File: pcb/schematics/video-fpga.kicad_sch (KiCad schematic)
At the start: 42 parts, among them U4 LCMXO2-7000HC-4TG144C, X1 ASV-xxxMHz

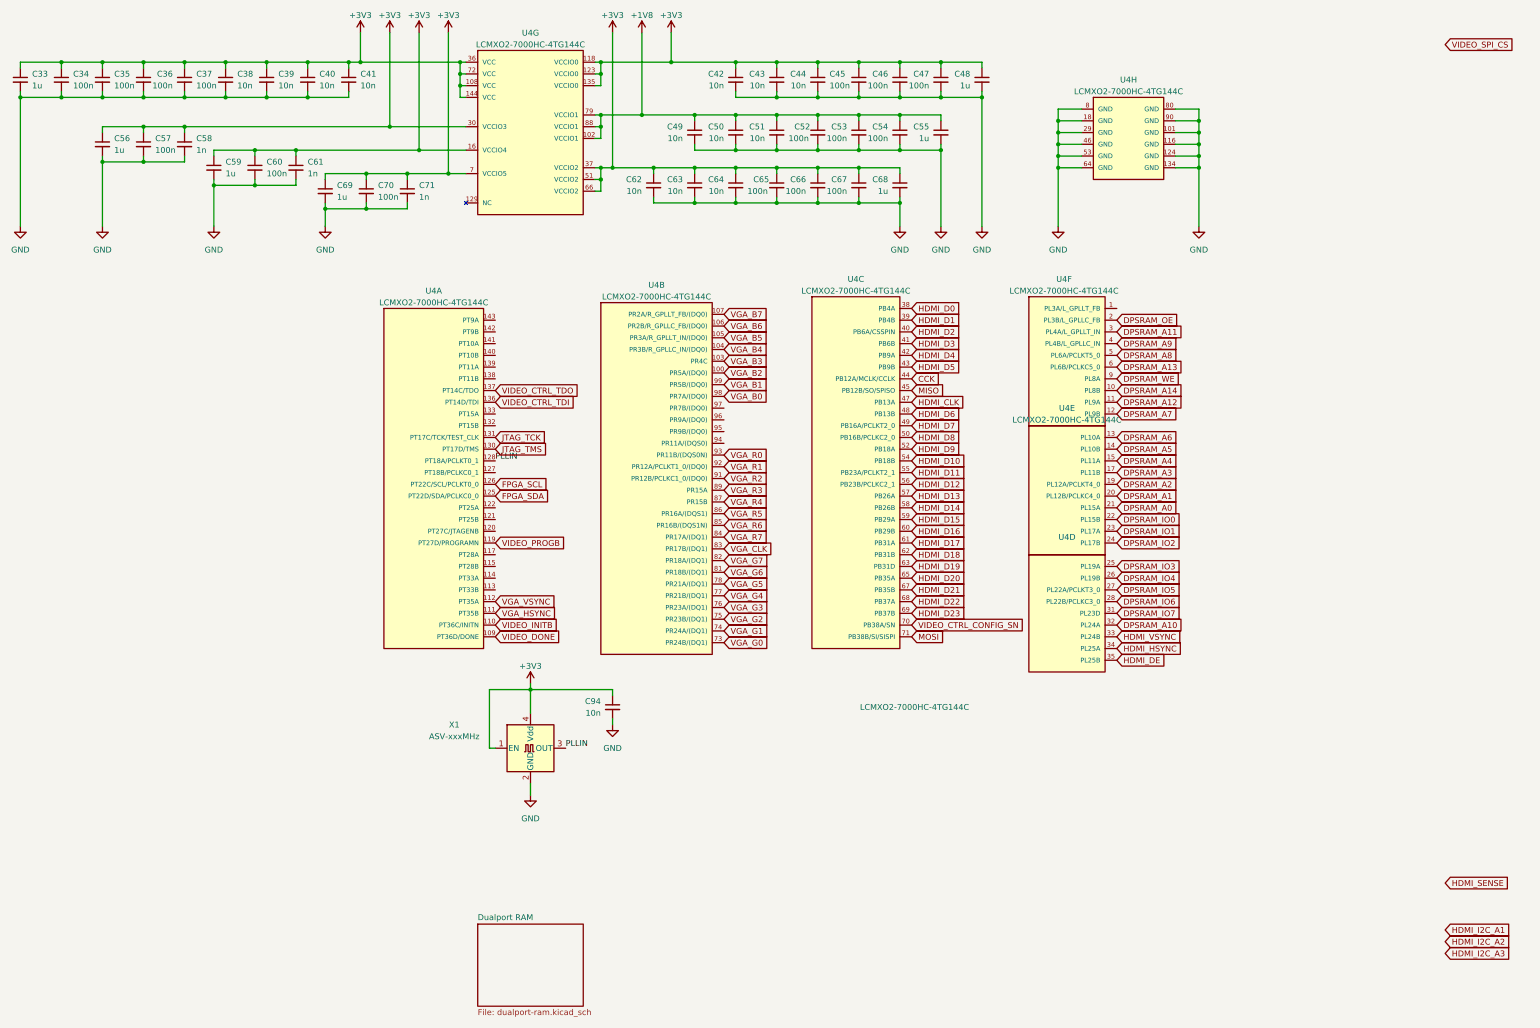
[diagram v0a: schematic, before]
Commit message: add shield
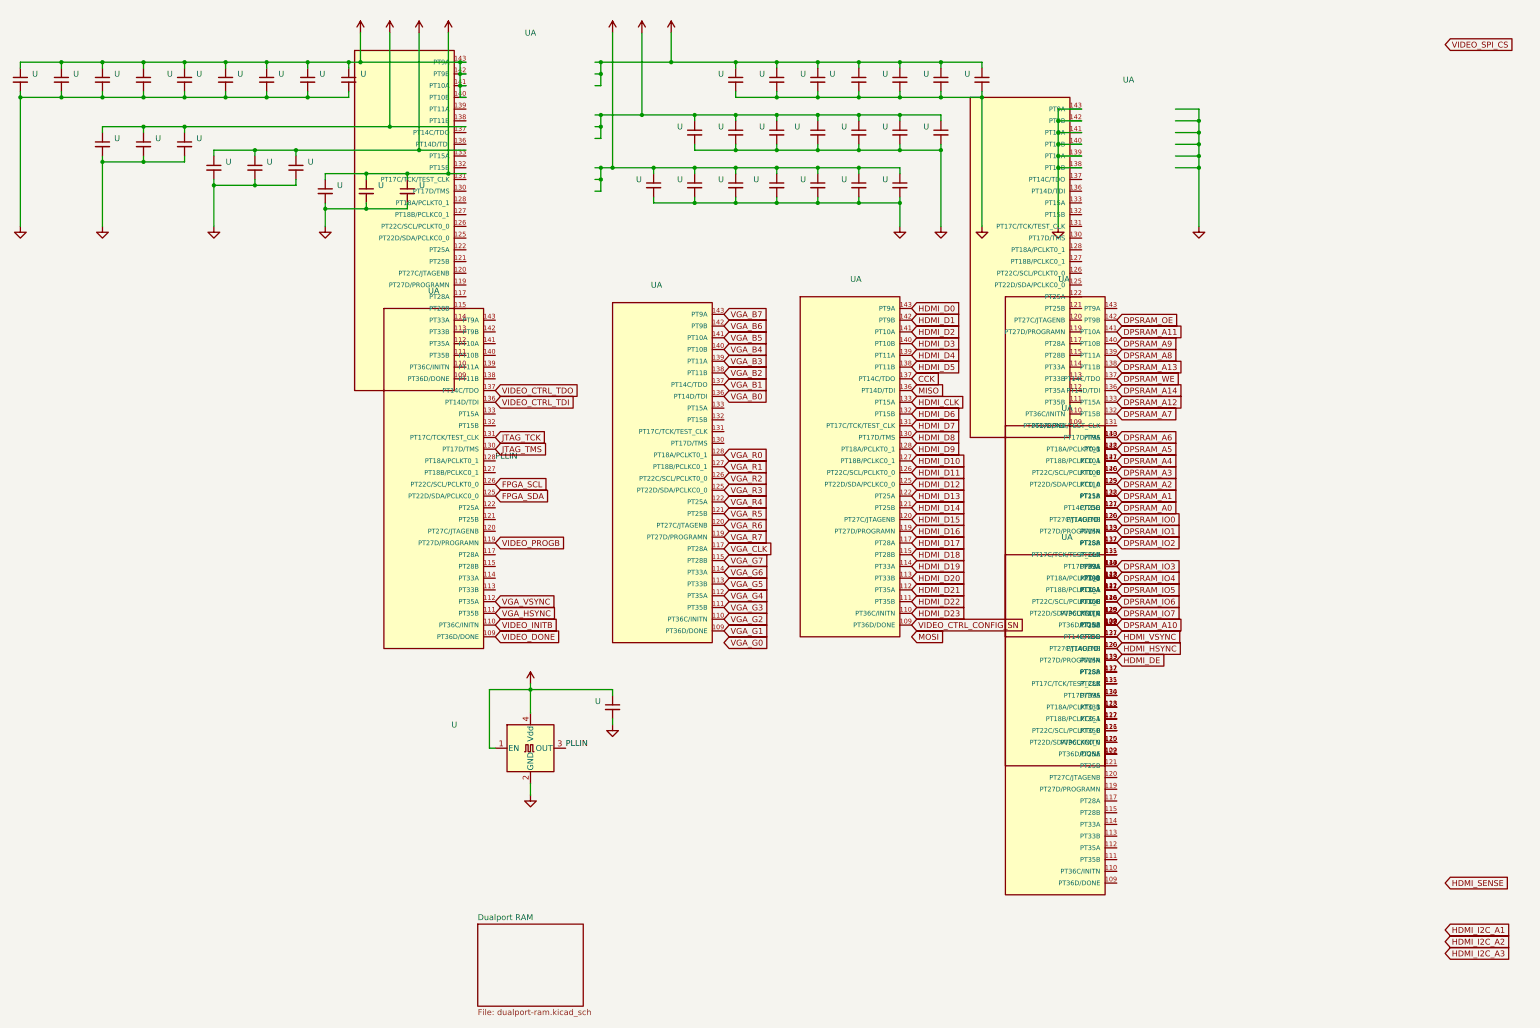
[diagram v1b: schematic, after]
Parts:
- U: renamed from C67; value 100n -> (none); footprint Capacitor_SMD:C_0603_1608Metric -> (none)
- U: renamed from U4; value LCMXO2-7000HC-4TG144C -> (none); footprint LCMXO2-7000HC-4TG144C:Lattice_Semiconductor-LCMXO2-7000HC-4TG144C-Level_C -> (none)
- U: renamed from C64; value 10n -> (none); footprint Capacitor_SMD:C_0402_1005Metric -> (none)
- U: renamed from C52; value 100n -> (none); footprint Capacitor_SMD:C_0603_1608Metric -> (none)
- U: renamed from C57; value 100n -> (none); footprint Capacitor_SMD:C_0603_1608Metric -> (none)
- U: renamed from C66; value 100n -> (none); footprint Capacitor_SMD:C_0603_1608Metric -> (none)
- U: renamed from C63; value 10n -> (none); footprint Capacitor_SMD:C_0402_1005Metric -> (none)
- U: renamed from C33; value 1u -> (none); footprint Capacitor_SMD:C_0805_2012Metric -> (none)
- U: renamed from C42; value 10n -> (none); footprint Capacitor_SMD:C_0402_1005Metric -> (none)
- U: renamed from C43; value 10n -> (none); footprint Capacitor_SMD:C_0402_1005Metric -> (none)
- U: renamed from C37; value 100n -> (none); footprint Capacitor_SMD:C_0603_1608Metric -> (none)
- U: renamed from C55; value 1u -> (none); footprint Capacitor_SMD:C_0805_2012Metric -> (none)
- U: renamed from C71; value 1n -> (none); footprint Capacitor_SMD:C_0402_1005Metric -> (none)
- U: renamed from C41; value 10n -> (none); footprint Capacitor_SMD:C_0402_1005Metric -> (none)
- U: renamed from C48; value 1u -> (none); footprint Capacitor_SMD:C_0805_2012Metric -> (none)
- U: renamed from C61; value 1n -> (none); footprint Capacitor_SMD:C_0402_1005Metric -> (none)
- U: renamed from C35; value 100n -> (none); footprint Capacitor_SMD:C_0603_1608Metric -> (none)
- U: renamed from C56; value 1u -> (none); footprint Capacitor_SMD:C_0805_2012Metric -> (none)
- U: renamed from C34; value 100n -> (none); footprint Capacitor_SMD:C_0603_1608Metric -> (none)
- U: renamed from C53; value 100n -> (none); footprint Capacitor_SMD:C_0603_1608Metric -> (none)
- U: renamed from C51; value 10n -> (none); footprint Capacitor_SMD:C_0402_1005Metric -> (none)
- U: renamed from C58; value 1n -> (none); footprint Capacitor_SMD:C_0402_1005Metric -> (none)
- U: renamed from C44; value 10n -> (none); footprint Capacitor_SMD:C_0402_1005Metric -> (none)
- U: renamed from C49; value 10n -> (none); footprint Capacitor_SMD:C_0402_1005Metric -> (none)
- U: renamed from C60; value 100n -> (none); footprint Capacitor_SMD:C_0603_1608Metric -> (none)
- U: renamed from C39; value 10n -> (none); footprint Capacitor_SMD:C_0402_1005Metric -> (none)
- U: renamed from C36; value 100n -> (none); footprint Capacitor_SMD:C_0603_1608Metric -> (none)
- U: renamed from C50; value 10n -> (none); footprint Capacitor_SMD:C_0402_1005Metric -> (none)
- U: renamed from C69; value 1u -> (none); footprint Capacitor_SMD:C_0805_2012Metric -> (none)
- U: renamed from C54; value 100n -> (none); footprint Capacitor_SMD:C_0603_1608Metric -> (none)
- U: renamed from C59; value 1u -> (none); footprint Capacitor_SMD:C_0805_2012Metric -> (none)
- U: renamed from C45; value 100n -> (none); footprint Capacitor_SMD:C_0603_1608Metric -> (none)
- U: renamed from C70; value 100n -> (none); footprint Capacitor_SMD:C_0603_1608Metric -> (none)
- U: renamed from C38; value 10n -> (none); footprint Capacitor_SMD:C_0402_1005Metric -> (none)
- U: renamed from C94; value 10n -> (none); footprint Capacitor_SMD:C_0402_1005Metric -> (none)
- U: renamed from X1; value ASV-xxxMHz -> (none); footprint Oscillator:Oscillator_SMD_Abracon_ASV-4Pin_7.0x5.1mm -> (none)
- U: renamed from C40; value 10n -> (none); footprint Capacitor_SMD:C_0402_1005Metric -> (none)
- U: renamed from C65; value 100n -> (none); footprint Capacitor_SMD:C_0603_1608Metric -> (none)
- U: renamed from C68; value 1u -> (none); footprint Capacitor_SMD:C_0805_2012Metric -> (none)
- U: renamed from C46; value 100n -> (none); footprint Capacitor_SMD:C_0603_1608Metric -> (none)
- U: renamed from C62; value 10n -> (none); footprint Capacitor_SMD:C_0402_1005Metric -> (none)
- U: renamed from C47; value 100n -> (none); footprint Capacitor_SMD:C_0603_1608Metric -> (none)
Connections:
- net +1V8: no longer U.102 (VCCIO1), U.79 (VCCIO1), U.88 (VCCIO1)
- net +3V3: now also U.140 (PT10B), U.141 (PT10A), U.142 (PT9B), U.143 (PT9A); no longer U.108 (VCC), U.118 (VCCIO0), U.123 (VCCIO0), U.135 (VCCIO0), U.144 (VCC), U.16 (VCCIO4), U.30 (VCCIO3), U.36 (VCC), U.37 (VCCIO2), U.51 (VCCIO2), U.66 (VCCIO2), U.7 (VCCIO5), U.72 (VCC)
- net CCK: now also U.137 (PT14C/TDO); no longer U.44 (PB12A/MCLK/CCLK)
- net DPSRAM_A0: now also U.121 (PT25B), U.137 (PT14C/TDO); no longer U.21 (PL15A)
- net DPSRAM_A1: now also U.122 (PT25A), U.138 (PT11B); no longer U.20 (PL12B/PCLKC4_0)
- net DPSRAM_A10: now also U.109 (PT36D/DONE), U.122 (PT25A), U.138 (PT11B); no longer U.32 (PL24A)
- net DPSRAM_A11: now also U.141 (PT10A); no longer U.3 (PL4A/L_GPLLT_IN)
- net DPSRAM_A12: now also U.133 (PT15A); no longer U.11 (PL9A)
- net DPSRAM_A13: now also U.138 (PT11B); no longer U.6 (PL6B/PCLKC5_0)
- net DPSRAM_A14: now also U.136 (PT14D/TDI); no longer U.10 (PL8B)
- net DPSRAM_A2: now also U.125 (PT22D/SDA/PCLKC0_0), U.139 (PT11A); no longer U.19 (PL12A/PCLKT4_0)
- net DPSRAM_A3: now also U.126 (PT22C/SCL/PCLKT0_0), U.140 (PT10B); no longer U.17 (PL11B)
- net DPSRAM_A4: now also U.127 (PT18B/PCLKC0_1), U.141 (PT10A); no longer U.15 (PL11A)
- net DPSRAM_A5: now also U.128 (PT18A/PCLKT0_1), U.142 (PT9B); no longer U.14 (PL10B)
- net DPSRAM_A6: now also U.130 (PT17D/TMS), U.143 (PT9A); no longer U.13 (PL10A)
- net DPSRAM_A7: now also U.132 (PT15B); no longer U.12 (PL9B)
- net DPSRAM_A8: now also U.139 (PT11A); no longer U.5 (PL6A/PCLKT5_0)
- net DPSRAM_A9: now also U.140 (PT10B); no longer U.4 (PL4B/L_GPLLC_IN)
- net DPSRAM_IO0: now also U.120 (PT27C/JTAGENB), U.136 (PT14D/TDI); no longer U.22 (PL15B)
- net DPSRAM_IO1: now also U.119 (PT27D/PROGRAMN), U.133 (PT15A); no longer U.23 (PL17A)
- net DPSRAM_IO2: now also U.117 (PT28A), U.132 (PT15B); no longer U.24 (PL17B)
- net DPSRAM_IO3: now also U.114 (PT33A), U.130 (PT17D/TMS), U.143 (PT9A); no longer U.25 (PL19A)
- net DPSRAM_IO4: now also U.113 (PT33B), U.128 (PT18A/PCLKT0_1), U.142 (PT9B); no longer U.26 (PL19B)
- net DPSRAM_IO5: now also U.112 (PT35A), U.127 (PT18B/PCLKC0_1), U.141 (PT10A); no longer U.27 (PL22A/PCLKT3_0)
- net DPSRAM_IO6: now also U.111 (PT35B), U.126 (PT22C/SCL/PCLKT0_0), U.140 (PT10B); no longer U.28 (PL22B/PCLKC3_0)
- net DPSRAM_IO7: now also U.110 (PT36C/INITN), U.125 (PT22D/SDA/PCLKC0_0), U.139 (PT11A); no longer U.31 (PL23D)
- net DPSRAM_OE: now also U.142 (PT9B); no longer U.2 (PL3B/L_GPLLC_FB)
- net DPSRAM_WE: now also U.137 (PT14C/TDO); no longer U.9 (PL8A)
- net GND: now also U.138 (PT11B), U.139 (PT11A), U.140 (PT10B), U.141 (PT10A), U.142 (PT9B), U.143 (PT9A); no longer U.101 (GND), U.116 (GND), U.124 (GND), U.134 (GND), U.18 (GND), U.29 (GND), U.46 (GND), U.53 (GND), U.64 (GND), U.8 (GND), U.80 (GND), U.90 (GND)
- net HDMI_CLK: now also U.133 (PT15A); no longer U.47 (PB13A)
- net HDMI_D0: now also U.143 (PT9A); no longer U.38 (PB4A)
- net HDMI_D1: now also U.142 (PT9B); no longer U.39 (PB4B)
- net HDMI_D10: now also U.127 (PT18B/PCLKC0_1); no longer U.54 (PB18B)
- net HDMI_D11: now also U.126 (PT22C/SCL/PCLKT0_0); no longer U.55 (PB23A/PCLKT2_1)
- net HDMI_D12: now also U.125 (PT22D/SDA/PCLKC0_0); no longer U.56 (PB23B/PCLKC2_1)
- net HDMI_D13: now also U.122 (PT25A); no longer U.57 (PB26A)
- net HDMI_D14: now also U.121 (PT25B); no longer U.58 (PB26B)
- net HDMI_D15: now also U.120 (PT27C/JTAGENB); no longer U.59 (PB29A)
- net HDMI_D16: now also U.119 (PT27D/PROGRAMN); no longer U.60 (PB29B)
- net HDMI_D17: now also U.117 (PT28A); no longer U.61 (PB31A)
- net HDMI_D18: now also U.115 (PT28B); no longer U.62 (PB31B)
- net HDMI_D19: now also U.114 (PT33A); no longer U.63 (PB31D)
- net HDMI_D2: now also U.141 (PT10A); no longer U.40 (PB6A/CSSPIN)
- net HDMI_D20: now also U.113 (PT33B); no longer U.65 (PB35A)
- net HDMI_D21: now also U.112 (PT35A); no longer U.67 (PB35B)
- net HDMI_D22: now also U.111 (PT35B); no longer U.68 (PB37A)
- net HDMI_D23: now also U.110 (PT36C/INITN); no longer U.69 (PB37B)
- net HDMI_D3: now also U.140 (PT10B); no longer U.41 (PB6B)
- net HDMI_D4: now also U.139 (PT11A); no longer U.42 (PB9A)
- net HDMI_D5: now also U.138 (PT11B); no longer U.43 (PB9B)
- net HDMI_D6: now also U.132 (PT15B); no longer U.48 (PB13B)
- net HDMI_D7: now also U.131 (PT17C/TCK/TEST_CLK); no longer U.49 (PB16A/PCLKT2_0)
- net HDMI_D8: now also U.130 (PT17D/TMS); no longer U.50 (PB16B/PCLKC2_0)
- net HDMI_D9: now also U.128 (PT18A/PCLKT0_1); no longer U.52 (PB18A)
- net HDMI_DE: now also U.119 (PT27D/PROGRAMN), U.133 (PT15A); no longer U.35 (PL25B)
- net HDMI_HSYNC: now also U.120 (PT27C/JTAGENB), U.136 (PT14D/TDI); no longer U.34 (PL25A)
- net HDMI_VSYNC: now also U.121 (PT25B), U.137 (PT14C/TDO); no longer U.33 (PL24B)
- net MISO: now also U.136 (PT14D/TDI); no longer U.45 (PB12B/SO/SPISO)
- net MOSI: no longer U.71 (PB38B/SI/SISPI)
- net VGA_B0: now also U.136 (PT14D/TDI); no longer U.98 (PR7A/(DQ0))
- net VGA_B1: now also U.137 (PT14C/TDO); no longer U.99 (PR5B/(DQ0))
- net VGA_B2: now also U.138 (PT11B); no longer U.100 (PR5A/(DQ0))
- net VGA_B3: now also U.139 (PT11A); no longer U.103 (PR4C)
- net VGA_B4: now also U.140 (PT10B); no longer U.104 (PR3B/R_GPLLC_IN/(DQ0))
- net VGA_B5: now also U.141 (PT10A); no longer U.105 (PR3A/R_GPLLT_IN/(DQ0))
- net VGA_B6: now also U.142 (PT9B); no longer U.106 (PR2B/R_GPLLC_FB/(DQ0))
- net VGA_B7: now also U.143 (PT9A); no longer U.107 (PR2A/R_GPLLT_FB/(DQ0))
- net VGA_CLK: now also U.117 (PT28A); no longer U.83 (PR17B/(DQ1))
- net VGA_G0: no longer U.73 (PR24B/(DQ1))
- net VGA_G1: now also U.109 (PT36D/DONE); no longer U.74 (PR24A/(DQ1))
- net VGA_G2: now also U.110 (PT36C/INITN); no longer U.75 (PR23B/(DQ1))
- net VGA_G3: now also U.111 (PT35B); no longer U.76 (PR23A/(DQ1))
- net VGA_G4: now also U.112 (PT35A); no longer U.77 (PR21B/(DQ1))
- net VGA_G5: now also U.113 (PT33B); no longer U.78 (PR21A/(DQ1))
- net VGA_G6: now also U.114 (PT33A); no longer U.81 (PR18B/(DQ1))
- net VGA_G7: now also U.115 (PT28B); no longer U.82 (PR18A/(DQ1))
- net VGA_R0: now also U.128 (PT18A/PCLKT0_1); no longer U.93 (PR11B/(DQS0N))
- net VGA_R1: now also U.127 (PT18B/PCLKC0_1); no longer U.92 (PR12A/PCLKT1_0/(DQ0))
- net VGA_R2: now also U.126 (PT22C/SCL/PCLKT0_0); no longer U.91 (PR12B/PCLKC1_0/(DQ0))
- net VGA_R3: now also U.125 (PT22D/SDA/PCLKC0_0); no longer U.89 (PR15A)
- net VGA_R4: now also U.122 (PT25A); no longer U.87 (PR15B)
- net VGA_R5: now also U.121 (PT25B); no longer U.86 (PR16A/(DQS1))
- net VGA_R6: now also U.120 (PT27C/JTAGENB); no longer U.85 (PR16B/(DQS1N))
- net VGA_R7: now also U.119 (PT27D/PROGRAMN); no longer U.84 (PR17A/(DQ1))
- net VIDEO_CTRL_CONFIG_SN: now also U.109 (PT36D/DONE); no longer U.70 (PB38A/SN)
- new net: U.109 (PT36D/DONE), U.122 (PT25A)
- new net: U.110 (PT36C/INITN), U.125 (PT22D/SDA/PCLKC0_0)
- new net: U.111 (PT35B), U.126 (PT22C/SCL/PCLKT0_0)
- new net: U.112 (PT35A), U.127 (PT18B/PCLKC0_1)
- new net: U.113 (PT33B), U.128 (PT18A/PCLKT0_1)
- new net: U.114 (PT33A), U.130 (PT17D/TMS)
- new net: U.115 (PT28B), U.131 (PT17C/TCK/TEST_CLK) (x2)
- new net: U.117 (PT28A), U.132 (PT15B)
